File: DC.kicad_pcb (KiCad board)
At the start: 4 copper layers, 196.5 x 181.5 mm, 87 parts, among them J1 348302001, J2 348302001, J3 757570141, J4 PPTC021LFBN-RC, U6 MCP2551-I-P, U7 NUCLEO-F302R8

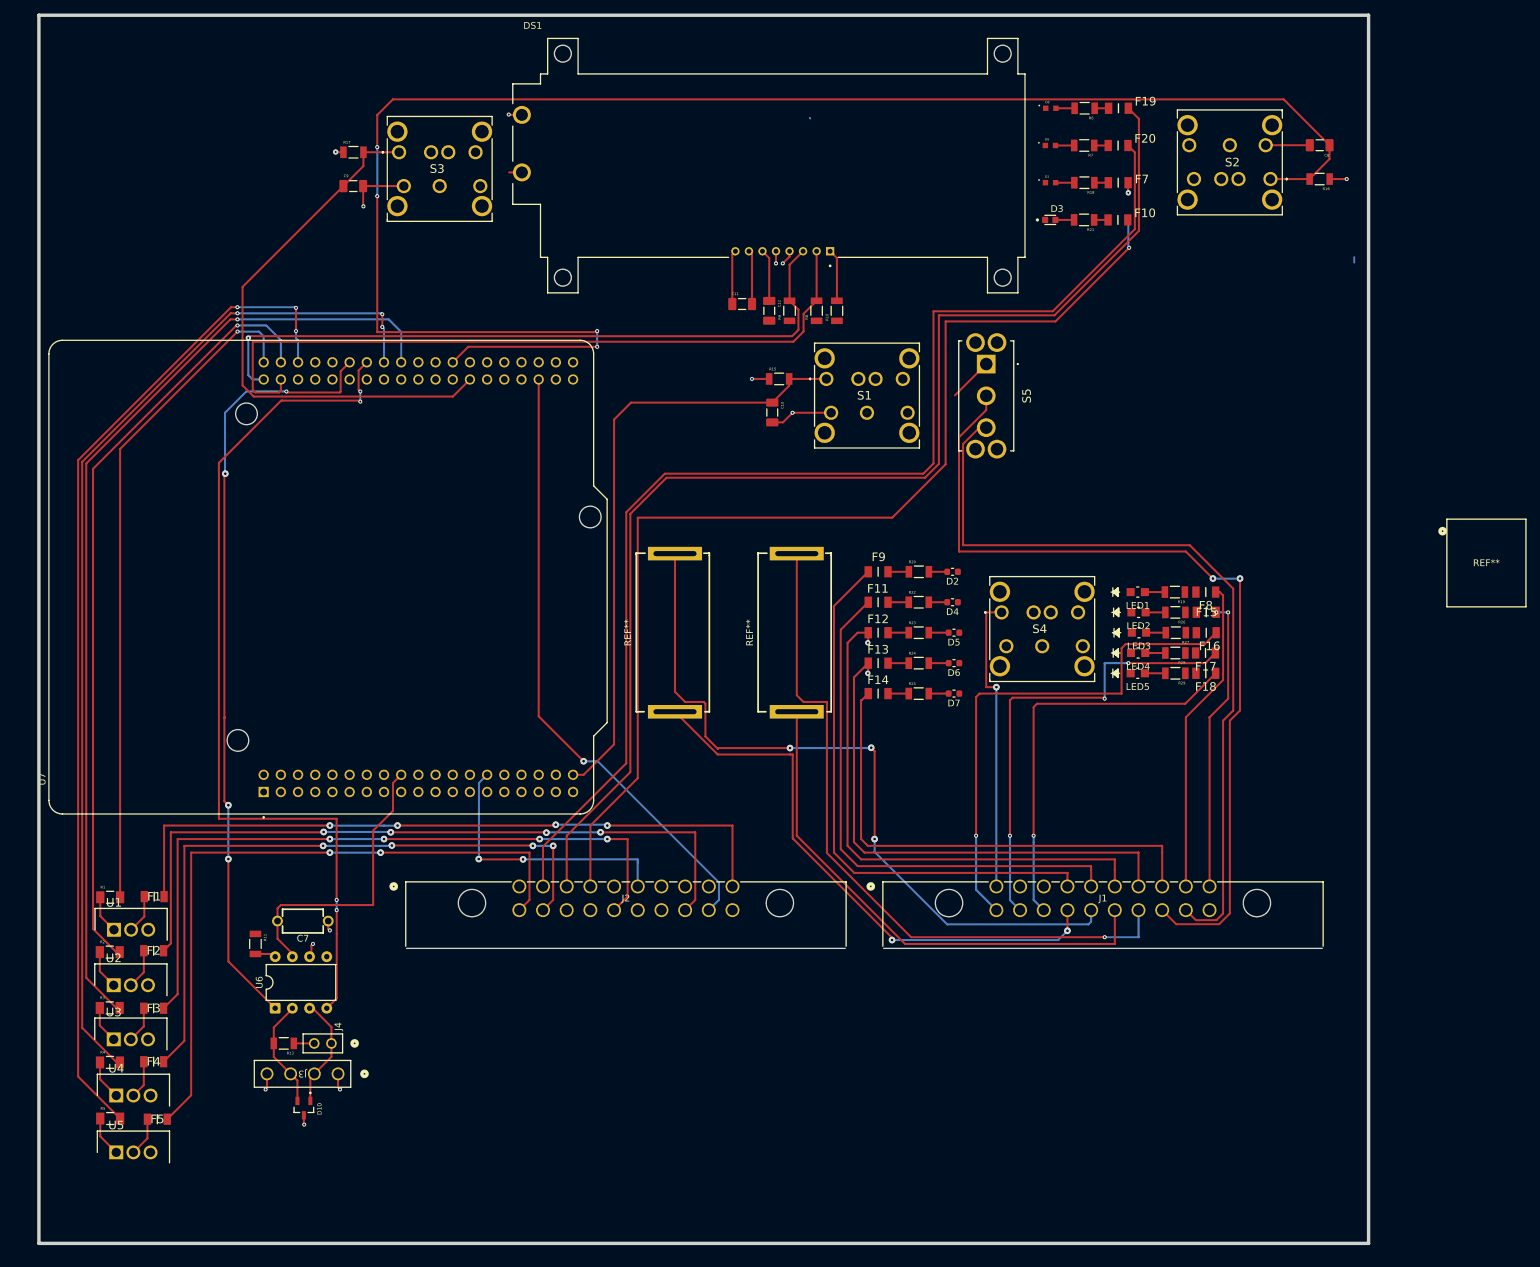
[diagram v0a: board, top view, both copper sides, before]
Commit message: Updated pcb with new routing and gear select. Still errors to correct
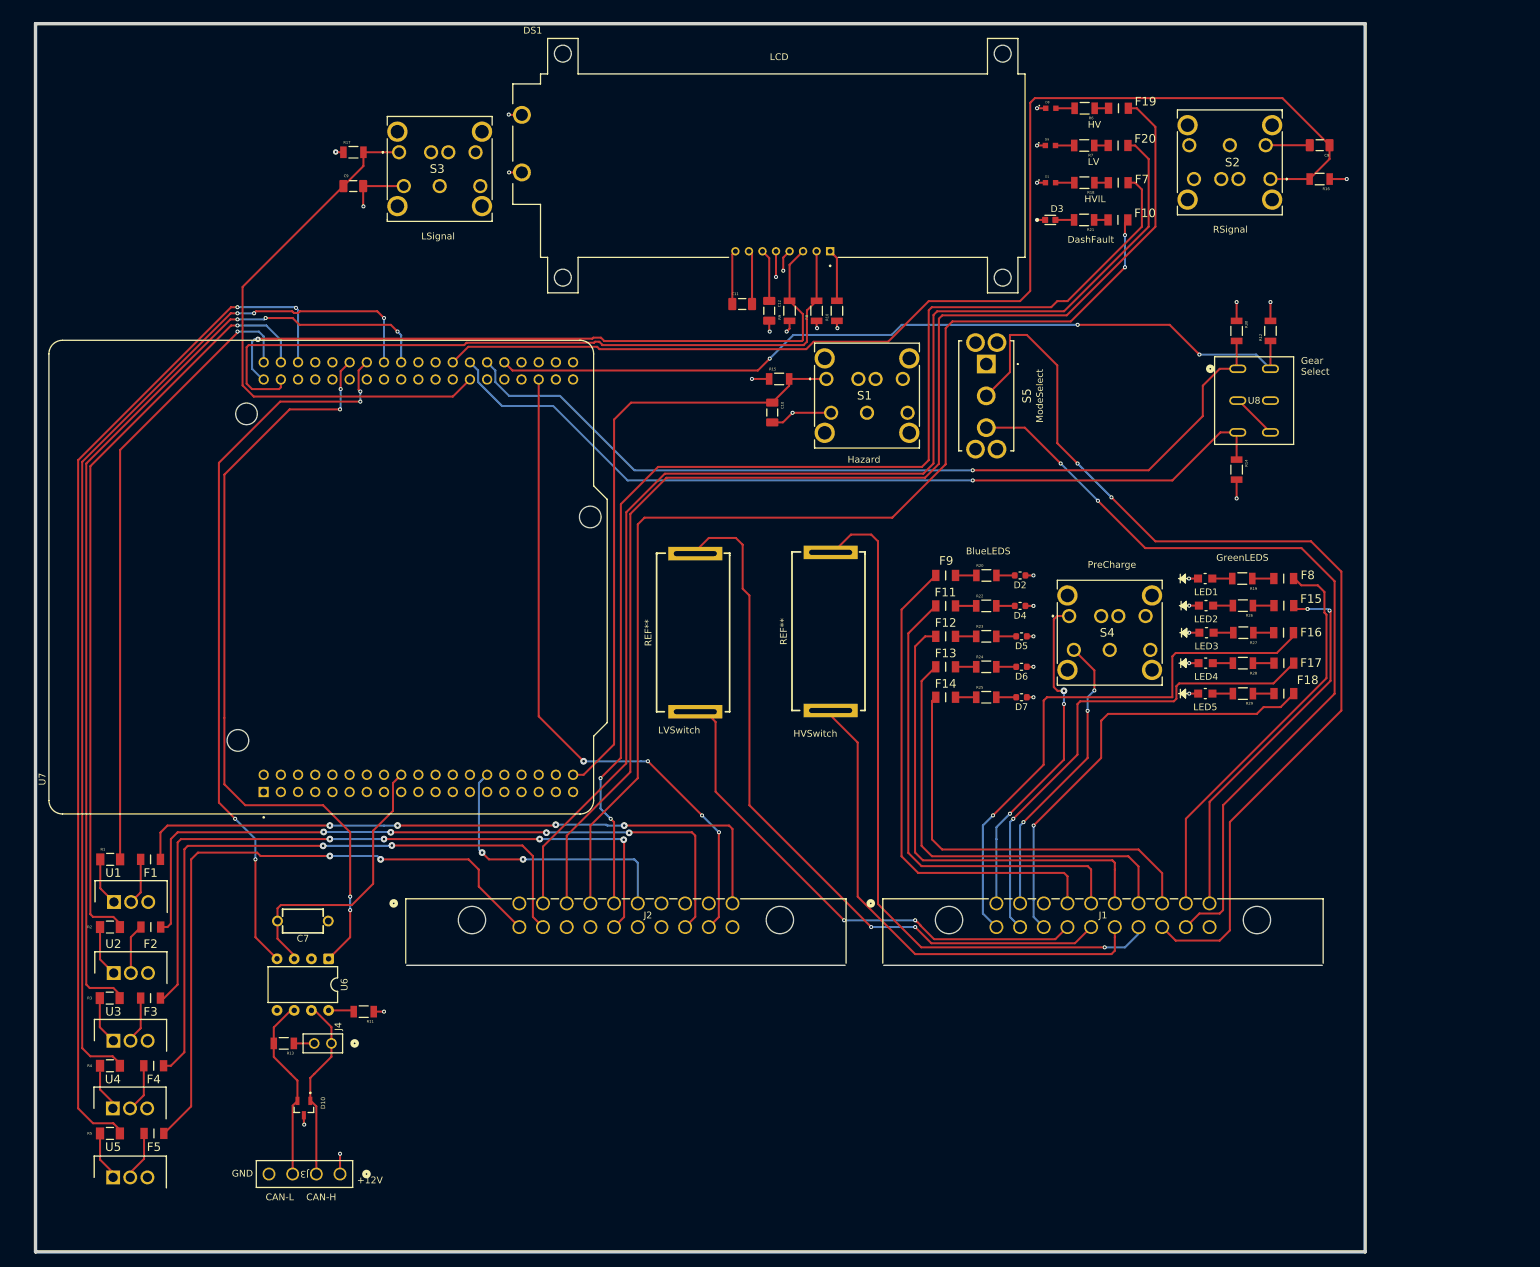
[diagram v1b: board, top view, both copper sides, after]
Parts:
- removed the REF** at (285.0, 92.0)
- added R12: RC1206FR-0710KL, MiscellaneousLibrary:RESC3116X65N, F.Cu at (255.5, 62.4)
- added R14: RC1206FR-0710KL, MiscellaneousLibrary:RESC3116X65N, F.Cu at (250.5, 82.9)
- added R30: RC1206FR-0710KL, MiscellaneousLibrary:RESC3116X65N, F.Cu at (250.5, 62.4)
- added U8: 100DP6T1B1M1QEH, MiscellaneousLibrary:TO_1M1QEH_EWI, F.Cu at (250.7, 68.0)
- moved R11 18.9 mm to (121.5, 163.0), turned to 180 degrees
- moved J3 14.8 mm to (118.0, 187.0)
- moved F18 11.9 mm to (257.5, 116.0)
- moved F8 11.7 mm to (257.5, 99.0)
- moved F17 11.7 mm to (257.5, 111.5)
- moved F15 11.5 mm to (257.5, 103.0)
- moved F16 11.4 mm to (257.4, 107.0)
- moved U6 10.8 mm to (116.3, 155.2), turned to -90 degrees
- moved LED5 10.4 mm to (245.9, 116.0)
- moved R29 10.4 mm to (251.4, 116.0)
- moved LED1 10.2 mm to (245.9, 99.0)
- moved R19 10.2 mm to (251.3, 99.0)
- moved LED4 10.1 mm to (245.9, 111.5)
- moved R28 10.1 mm to (251.4, 111.5)
- moved R26 10.0 mm to (251.4, 103.0)
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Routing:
- net /HVILActive: track 1.52 -> 176.0 mm, vias 1 -> 2
- net /Neutral: track 0.00 -> 131.6 mm, vias 0 -> 1
- net /Drive: track 0.00 -> 128.7 mm, vias 0 -> 1
- net /Reverse: track 0.00 -> 123.3 mm, vias 0 -> 3
- net /RSignalLightIn: track 245.8 -> 177.2 mm, vias 4 -> 0
- net /From_PreChargeBtn: track 0.00 -> 43.3 mm, vias 0 -> 3
- net /To_ModeSelect: track 129.5 -> 151.9 mm
- net /CAN_RX: track 129.8 -> 108.2 mm
- net GND: track 35.3 -> 49.8 mm, vias 7 -> 22
- net /GreenLED1: track 46.6 -> 60.1 mm
- net /GreenLED2: track 43.4 -> 56.3 mm
- net +3.3V: track 9.92 -> 22.4 mm, vias 4 -> 10
- net /BlueLED5: track 72.9 -> 61.8 mm
- net /CAN_H: track 16.4 -> 27.1 mm
- net /BlueLED4: track 76.5 -> 66.1 mm, vias 1 -> 0
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- added copper zone on In1.Cu, net +3.3V
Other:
- board text added: "+12V"
- board text added: "BlueLEDS"
- board text added: "CAN-H"
- board text added: "CAN-L"
- board text added: "DashFault"
- board text added: "GND"
- board text added: "Gear Select"
- board text added: "GreenLEDS"
- board text added: "HV"
- board text added: "HVIL"
- board text added: "HVSwitch"
- board text added: "Hazard"
- board text added: "LCD"
- board text added: "LSignal"
- board text added: "LV"
- board text added: "LVSwitch"
- board text added: "ModeSelect"
- board text added: "PreCharge"
- board text added: "RSignal"

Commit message: VCU revisions, last review still to be done
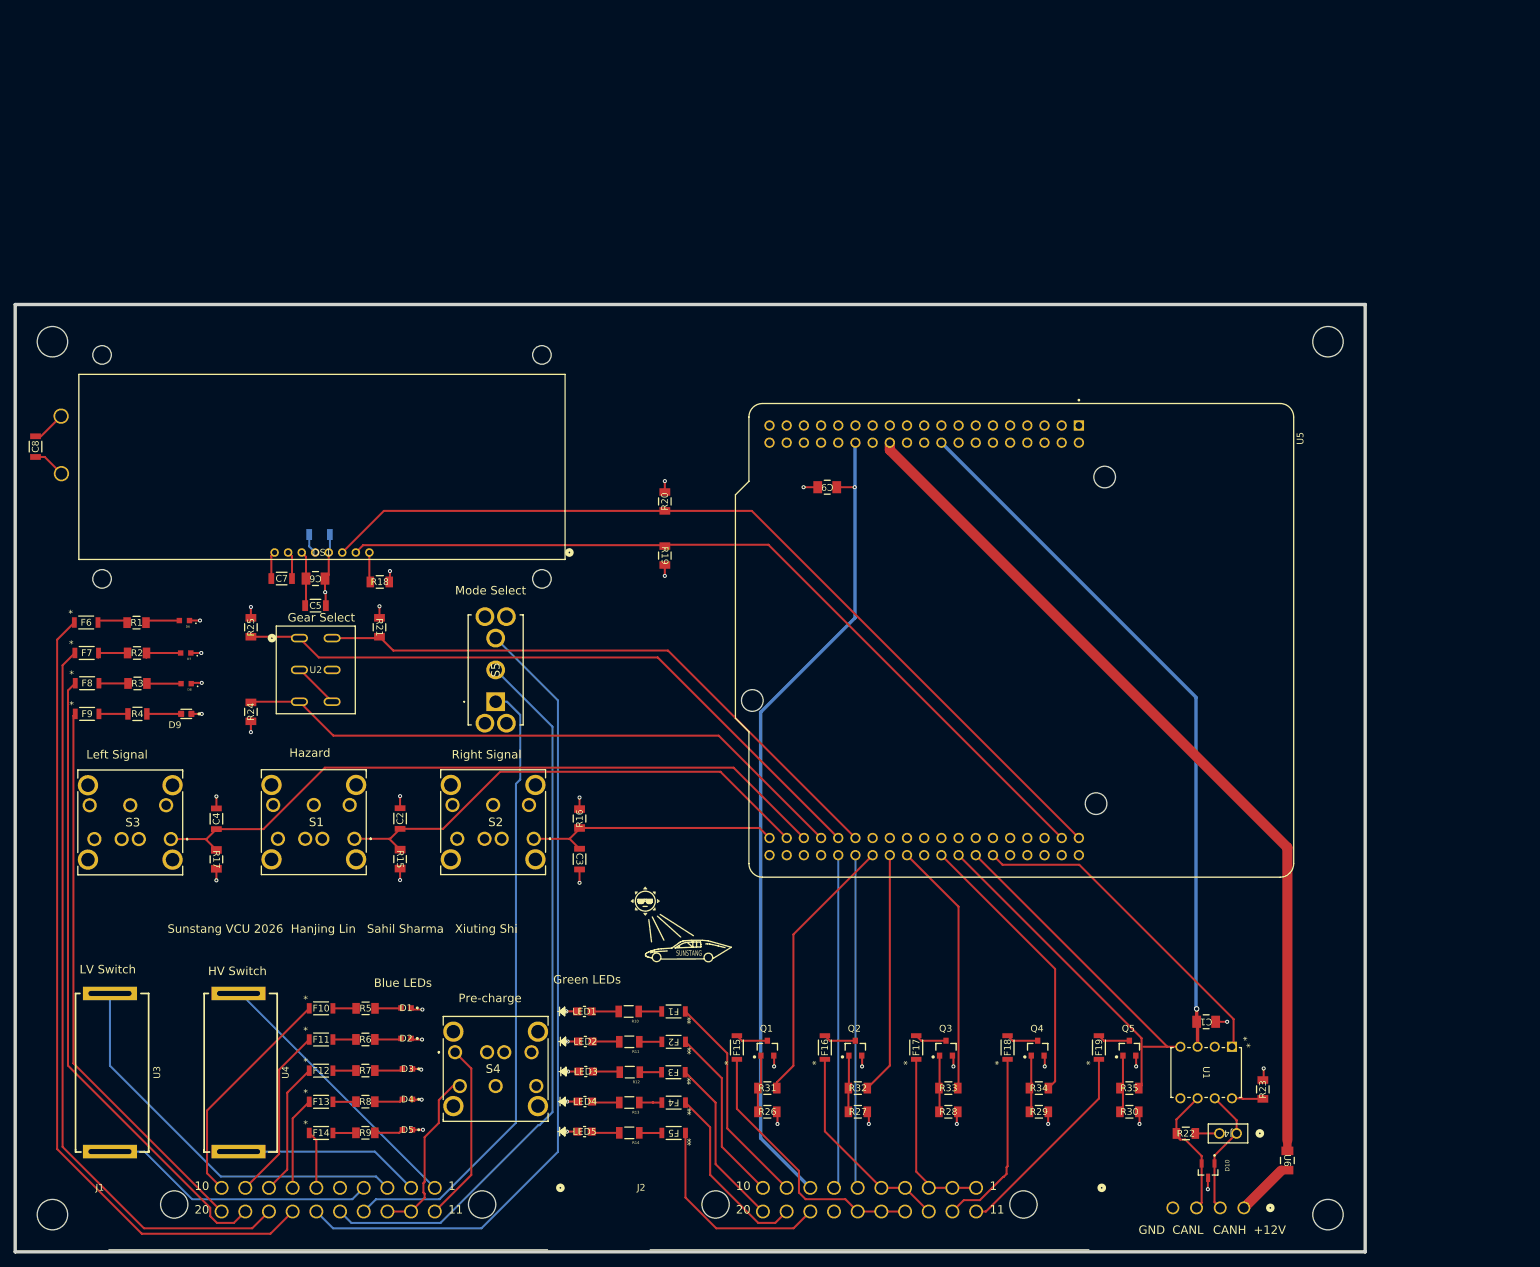
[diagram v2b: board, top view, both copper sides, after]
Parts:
- removed C11: CL31B105KAHNNNE, Capacitor_SMD:CAPC3216X180N
- removed C12: C3216X7R2A474K160AA, Capacitor_SMD:CAPC3216X180N
- removed the F1 at (90.0, 140.5)
- removed the F2 at (90.0, 150.5)
- removed the F3 at (90.0, 161.0)
- removed the F4 at (90.5, 171.0)
- removed the F5 at (90.5, 181.0)
- removed the R18 at (228.0, 40.5)
- removed the R4 at (84.0, 171.0)
- removed the R5 at (84.0, 181.0)
- removed the R6 at (228.0, 29.5)
- removed the R7 at (228.0, 35.0)
- removed the REF** at (170.5, 107.0)
- removed the REF** at (190.5, 106.8)
- removed the U1 at (84.6, 146.8)
- removed the U5 at (84.5, 187.5)
- removed U8: 100DP6T1B1M1QEH, MiscellaneousLibrary:TO_1M1QEH_EWI
- added C1: C1206C104K5RACTU, DriverControlsLib:CAPC340180_88N_KEM, F.Cu at (246.0, 164.5)
- added C5: CL31B105KAHNNNE, DriverControlsLib:CAP_CL31_SAM, F.Cu at (114.4, 103.0)
- added C6: C1206C104K5RACTU, DriverControlsLib:CAPC340180_88N_KEM, F.Cu at (114.4, 99.0)
- added C8: CL31B225KBHNNNE, DriverControlsLib:CAP_CL31_SAM, F.Cu at (73.0, 79.5)
- added C8: CL31B225KBHNNNE, DriverControlsLib:CAP_CL31_SAM, B.Cu at (115.0, 92.5)
- added C9: C1206C104K5RACTU, DriverControlsLib:CAPC340180_88N_KEM, F.Cu at (190.0, 85.5)
- added F15: 0466.125NR, DriverControlsLib:0466Series_LTF, F.Cu at (176.7, 168.3)
- added F16: 0466.125NR, DriverControlsLib:0466Series_LTF, F.Cu at (189.7, 168.3)
- added F17: 0466.125NR, DriverControlsLib:0466Series_LTF, F.Cu at (203.2, 168.3)
- added F18: 0466.125NR, DriverControlsLib:0466Series_LTF, F.Cu at (216.7, 168.3)
- added F19: 0466.125NR, DriverControlsLib:0466Series_LTF, F.Cu at (230.2, 168.3)
- added Q1: BSS806NE, DriverControlsLib:SOT95P240X110-3N-1-V1, F.Cu at (181.2, 168.4)
- added Q2: BSS806NE, DriverControlsLib:SOT95P240X110-3N-1-V1, F.Cu at (194.2, 168.4)
- added Q3: BSS806NE, DriverControlsLib:SOT95P240X110-3N-1-V1, F.Cu at (207.6, 168.4)
- added Q4: BSS806NE, DriverControlsLib:SOT95P240X110-3N-1-V1, F.Cu at (221.1, 168.4)
- added Q5: BSS806NE, DriverControlsLib:SOT95P240X110-3N-1-V1, F.Cu at (234.7, 168.4)
- added R26: RC1206FR-0710KL, DriverControlsLib:RC1206N_YAG, F.Cu at (181.2, 177.8)
- added R27: RC1206FR-0710KL, DriverControlsLib:RC1206N_YAG, F.Cu at (194.5, 177.8)
- added R28: RC1206FR-0710KL, DriverControlsLib:RC1206N_YAG, F.Cu at (207.9, 177.8)
- added R29: RC1206FR-0710KL, DriverControlsLib:RC1206N_YAG, F.Cu at (221.3, 177.8)
- added R30: RC1206FR-0710KL, DriverControlsLib:RC1206N_YAG, F.Cu at (234.7, 177.8)
- added R31: RC1206JR-07120RL, DriverControlsLib:RC1206N_YAG, F.Cu at (181.2, 174.3)
- added R32: RC1206JR-07120RL, DriverControlsLib:RC1206N_YAG, F.Cu at (194.5, 174.3)
- added R33: RC1206JR-07120RL, DriverControlsLib:RC1206N_YAG, F.Cu at (207.9, 174.3)
- added R34: RC1206JR-07120RL, DriverControlsLib:RC1206N_YAG, F.Cu at (221.3, 174.3)
- added R35: RC1206JR-07120RL, DriverControlsLib:RC1206N_YAG, F.Cu at (234.7, 174.3)
- added REF**: MountingHole_4.5mm, MountingHole:MountingHole_4.5mm, F.Cu at (264.0, 64.0)
- added REF**: MountingHole_4.5mm, MountingHole:MountingHole_4.5mm, F.Cu at (75.5, 193.0)
- added REF**: MountingHole_4.5mm, MountingHole:MountingHole_4.5mm, F.Cu at (264.0, 193.0)
- added REF**: MountingHole_4.5mm, MountingHole:MountingHole_4.5mm, F.Cu at (75.5, 64.0)
- added U6: C1F 3, DriverControlsLib:C1_BEL, F.Cu at (258.0, 185.0)
- C2: renamed from C10; footprint Capacitor_SMD:CAPC3216X180N -> DriverControlsLib:CAP_CL31_SAM
- C3: renamed from C8; footprint Capacitor_SMD:CAPC3216X180N -> DriverControlsLib:CAP_CL31_SAM
- C4: renamed from C9; footprint Capacitor_SMD:CAPC3216X180N -> DriverControlsLib:CAP_CL31_SAM
- C7: value C -> CL31B105KAHNNNE; footprint DriverControlsLib:CAP-TH_L6.0-W3.5-P7.50-D1.0 -> DriverControlsLib:CAP_CL31_SAM
- D1: renamed from D2; footprint Fuse:Fuse_0603_1608Metric -> DriverControlsLib:LED_LTST-C_LTO
- D2: renamed from D4; footprint Fuse:Fuse_0603_1608Metric -> DriverControlsLib:LED_LTST-C_LTO
- D3: renamed from D5; footprint Fuse:Fuse_0603_1608Metric -> DriverControlsLib:LED_LTST-C_LTO
- D4: renamed from D6; footprint Fuse:Fuse_0603_1608Metric -> DriverControlsLib:LED_LTST-C_LTO
- D5: renamed from D7; footprint Fuse:Fuse_0603_1608Metric -> DriverControlsLib:LED_LTST-C_LTO
- D6: renamed from D9; footprint LED_SMD:LEDM1608X80 -> DriverControlsLib:LEDM1608X80
- D7: renamed from D8; footprint LED_SMD:LEDM1608X80 -> DriverControlsLib:LEDM1608X80
- D8: renamed from D1; footprint LED_SMD:LEDM1608X80 -> DriverControlsLib:LEDM1608X80
- D9: renamed from D3; footprint LED_SMD:LEDC1608X65N -> DriverControlsLib:LEDC1608X65N
- DS1: footprint Display:LCD_NHD-C0220BIZ-FSW-FBW-3V3M -> DriverControlsLib:NHD-C0220BIZ-FSW-FBW-3V3M_NDI
- F1: renamed from F8; footprint Fuse:FUSC3215X66N -> DriverControlsLib:0466Series_LTF
- F10: renamed from F9; footprint Fuse:FUSC3215X66N -> DriverControlsLib:0466Series_LTF
- F11, F12, F13, F14: footprint Fuse:FUSC3215X66N -> DriverControlsLib:0466Series_LTF
- F2: renamed from F15; footprint Fuse:FUSC3215X66N -> DriverControlsLib:0466Series_LTF
- F3: renamed from F16; footprint Fuse:FUSC3215X66N -> DriverControlsLib:0466Series_LTF
- F4: renamed from F17; footprint Fuse:FUSC3215X66N -> DriverControlsLib:0466Series_LTF
- F5: renamed from F18; footprint Fuse:FUSC3215X66N -> DriverControlsLib:0466Series_LTF
- F6: renamed from F20; footprint Fuse:FUSC3215X66N -> DriverControlsLib:0466Series_LTF
- F7: renamed from F19; footprint Fuse:FUSC3215X66N -> DriverControlsLib:0466Series_LTF
- F8: renamed from F7; footprint Fuse:FUSC3215X66N -> DriverControlsLib:0466Series_LTF
- F9: renamed from F10; footprint Fuse:FUSC3215X66N -> DriverControlsLib:0466Series_LTF
- J1, J2: footprint Connector_Molex:CONN_SD-34829-001_20_ST_MOL -> DriverControlsLib:CONN_SD-34829-001_20_ST_MOL; moved to B.Cu
- J3: footprint Connector_Molex:CONN_SD-75757-010_1X4_F11p20_MOL -> DriverControlsLib:CONN_SD-75757-010_1X4_F11p20_MOL; moved to B.Cu
- J4: footprint Connector:CONN2_LFBN-RC_SUL -> DriverControlsLib:CONN2_LFBN-RC_SUL
- LED1, LED2, LED3, LED4, LED5: footprint LED_SMD:LED_LTST-C170GKT_LTO -> DriverControlsLib:LED_LTST-C170GKT_LTO
- R1, R2, R3: value 220Ω -> RC1206FR-07665RL; footprint Resistor_SMD:RESC3216X70N -> DriverControlsLib:RC1206N_YAG
- R10: renamed from R19; footprint Resistor_SMD:RESC3116X65N -> DriverControlsLib:RESC3116X65N
- R11: renamed from R26; footprint Resistor_SMD:RESC3116X65N -> DriverControlsLib:RESC3116X65N
- R12: renamed from R27; footprint Resistor_SMD:RESC3116X65N -> DriverControlsLib:RESC3116X65N
- R13: renamed from R28; footprint Resistor_SMD:RESC3116X65N -> DriverControlsLib:RESC3116X65N
- R14: renamed from R29; footprint Resistor_SMD:RESC3116X65N -> DriverControlsLib:RESC3116X65N
- R15, R16, R17: footprint Resistor_SMD:RESC3116X65N -> DriverControlsLib:RC1206N_YAG
- R18: renamed from R10; footprint Resistor_SMD:RESC3116X65N -> DriverControlsLib:RC1206N_YAG
- R19: renamed from R8; footprint Resistor_SMD:RESC3116X65N -> DriverControlsLib:RC1206N_YAG
- R20: renamed from R9; footprint Resistor_SMD:RESC3116X65N -> DriverControlsLib:RC1206N_YAG
- R21: renamed from R12; footprint MiscellaneousLibrary:RESC3116X65N -> DriverControlsLib:RC1206N_YAG
- R22: renamed from R13; footprint Resistor_SMD:RESC3116X65N -> DriverControlsLib:RC1206N_YAG
- R23: renamed from R11; footprint Resistor_SMD:RESC3116X65N -> DriverControlsLib:RC1206N_YAG
- R24: renamed from R14; footprint MiscellaneousLibrary:RESC3116X65N -> DriverControlsLib:RC1206N_YAG
- R25: renamed from R30; footprint MiscellaneousLibrary:RESC3116X65N -> DriverControlsLib:RC1206N_YAG
- R4: renamed from R21; footprint Resistor_SMD:RESC3116X65N -> DriverControlsLib:RES_RC1206_YAG
- R5: renamed from R20; footprint Resistor_SMD:RESC3116X65N -> DriverControlsLib:RC1206N_YAG
- R6: renamed from R22; footprint Resistor_SMD:RESC3116X65N -> DriverControlsLib:RC1206N_YAG
- R7: renamed from R23; footprint Resistor_SMD:RESC3116X65N -> DriverControlsLib:RC1206N_YAG
- R8: renamed from R24; footprint Resistor_SMD:RESC3116X65N -> DriverControlsLib:RC1206N_YAG
- R9: renamed from R25; footprint Resistor_SMD:RESC3116X65N -> DriverControlsLib:RC1206N_YAG
- S1, S2, S3, S4: footprint Button_Switch_SMD:LP6OA2ASRG -> DriverControlsLib:LP6OA2ASRG
- S5: footprint Button_Switch_SMD:100SP1T8B13VS2REH -> DriverControlsLib:100SP1T8B13VS2REH
- U1: renamed from U6; footprint Package_DIP:DIP-8_W7.62mm -> DriverControlsLib:PDIP8_300MC_MCH
- U2: value ~ -> 100DP6T1B1M1QEH; footprint Battery:TO254P470X1016X2019-3P -> DriverControlsLib:TO_1M1QEH_EWI
- U3: footprint Battery:TO254P470X1016X2019-3P -> DriverControlsLib:LV_Switch
- U4: footprint Battery:TO254P470X1016X2019-3P -> DriverControlsLib:HV_Switch
- U5: renamed from U7; footprint Module:MODULE_NUCLEO-F302R8 -> DriverControlsLib:MODULE_NUCLEO-F302R8
- moved F7 172.4 mm to (80.6, 110.0), turned to 0 degrees
- moved F8 169.4 mm to (80.6, 114.5), turned to 0 degrees
- moved F9 168.9 mm to (80.6, 119.0), turned to 0 degrees
- moved F6 168.0 mm to (80.5, 105.5), turned to 0 degrees
- moved R4 157.8 mm to (88.1, 119.0), turned to 0 degrees
- moved R25 152.1 mm to (104.8, 106.2), turned to 90 degrees
- moved C3 152.0 mm to (153.4, 140.5), turned to -90 degrees
- moved D7 151.1 mm to (95.2, 110.0), turned to 180 degrees
- moved R24 150.0 mm to (104.8, 118.7), turned to 90 degrees
- moved D8 147.6 mm to (95.3, 114.5), turned to 180 degrees
- moved D9 147.1 mm to (95.3, 119.0), turned to 180 degrees
- moved S2 146.2 mm to (146.6, 137.5)
- moved D6 146.0 mm to (95.0, 105.2), turned to 180 degrees
- moved R16 144.5 mm to (153.4, 134.5), turned to 90 degrees
- moved R21 138.8 mm to (123.8, 106.2), turned to -90 degrees
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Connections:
- C7 pad 1: GND -> Net-(DS1-C1-)
- C7 pad 2: /CANTransceiver5V -> Net-(DS1-C1+)
- D1 pad 2: Net-(D2-Pad2) -> Net-(D1-Pad2)
- D2 pad 2: Net-(D4-Pad2) -> Net-(D2-Pad2)
- D3 pad 2: Net-(D5-Pad2) -> Net-(D3-Pad2)
- D4 pad 2: Net-(D6-Pad2) -> Net-(D4-Pad2)
- D5 pad 2: Net-(D7-Pad2) -> Net-(D5-Pad2)
- D6 pad A: Net-(D9-PadA) (its old number) -> Net-(D6-PadA)
- D7 pad A: Net-(D8-PadA) -> Net-(D7-PadA)
- D8 pad A: Net-(D1-PadA) -> Net-(D8-PadA)
- DS1 pad 1: Net-(DS1A-RST) -> Net-(DS1-ST)
- DS1 pad 7: Net-(DS1A-C1P) -> Net-(DS1-C1+)
- DS1 pad 8: Net-(DS1A-C1N) -> Net-(DS1-C1-)
- F10 pad 2: Net-(F9-Pad2) (its old number) -> Net-(F10-Pad2)
- F6 pad 2: Net-(F20-Pad2) -> Net-(F6-Pad2)
- F7 pad 2: Net-(F19-Pad2) -> Net-(F7-Pad2)
- F8 pad 2: Net-(F7-Pad2) -> Net-(F8-Pad2)
- J1 pad 1: /To_PreChargeBtn -> /HVSwitch+
- J1 pad 10: /GreenLED2 -> /BlueLED1
- J1 pad 11: /GreenLED3 -> /To_PreChargeBtn
- J1 pad 12: /GreenLED4 -> /Enable
- J1 pad 13: /GreenLED5 -> /Enable
- J1 pad 14: /LVSwitch+ -> /ChargeMode
- J1 pad 15: /LVSwitch- -> /To_ModeSelect
- J1 pad 16: /HVSwitch+ -> /ReadyMode
- J1 pad 17: /HVSwitch- -> /LVActive
- J1 pad 18: /To_ModeSelect -> /HVActive
- J1 pad 19: /ReadyMode -> /HVILActive
- J1 pad 2: /From_PreChargeBtn -> /HVSwitch-
- J1 pad 20: GND -> /DashFaultIndicator
- J1 pad 3: /Enable -> /LVSwitch+
- J1 pad 4: /BlueLED1 -> /LVSwitch-
- J1 pad 5: /BlueLED2 -> GND
- J1 pad 6: /BlueLED3 -> /BlueLED5
- J1 pad 8: /BlueLED5 -> /BlueLED3
- J1 pad 9: /GreenLED1 -> /BlueLED2
- J2 pad 1: /ChargeMode -> /LSignalLightNeg
- J2 pad 10: /BrakeLightNeg -> /GreenLED2
- J2 pad 13: /LSignalLightNeg -> /RSignalLightNeg
- J2 pad 14: /LSignalLightNeg -> /BrakeLightNeg
- J2 pad 15: /LSignalLightNeg -> /BrakeLightNeg
- J2 pad 16: /RSignalLightNeg -> /BrakeLightNeg
- J2 pad 17: /RSignalLightNeg -> GND
- J2 pad 18: /RSignalLightNeg -> /GreenLED5
- J2 pad 19: /ThermalShutoff -> /GreenLED4
- J2 pad 2: /LVActive -> /LSignalLightNeg
- J2 pad 20: GND -> /GreenLED3
- J2 pad 3: /HVActive -> /LSignalLightNeg
- J2 pad 4: /DashFaultIndicator -> /RSignalLightNeg
- J2 pad 5: /HVILActive -> /RSignalLightNeg
- J2 pad 6: /AccelIn -> /ThermalShutoff
- J2 pad 7: /BrakeLightIn -> /BrakePedalIn
- J2 pad 8: /BrakeLightNeg -> /AccelIn
- J2 pad 9: /BrakeLightNeg -> /GreenLED1
- R1 pad 1: Net-(U1-G) -> Net-(D6-PadA)
- R1 pad 2: /BrakeLightOut -> Net-(F6-Pad2)
- R15 pad 1: +3.3V -> /HazardIn
- R15 pad 2: /HazardIn -> +3.3V
- R16 pad 1: +3.3V -> /RSignalLightIn
- R16 pad 2: /RSignalLightIn -> +3.3V
- R17 pad 1: +3.3V -> /LSignalLightIn
- R17 pad 2: /LSignalLightIn -> +3.3V
- R18 pad 1: GND -> Net-(DS1-ST)
- R18 pad 2: Net-(DS1A-RST) -> GND
- R19 pad 1: +3.3V -> /I2C1_CLK
- R19 pad 2: /I2C1_CLK -> +3.3V
- R2 pad 1: Net-(U2-G) -> Net-(D7-PadA)
- R2 pad 2: /RSignalLightOut -> Net-(F7-Pad2)
- R20 pad 1: +3.3V -> /I2C1_SDA
- R20 pad 2: /I2C1_SDA -> +3.3V
- R21 pad 1: /Reverse -> +3.3V
- R21 pad 2: +3.3V -> /Reverse
- R22 pad 1: Net-(J4-Pad2) -> /CAN_L
- R22 pad 2: /CAN_L -> Net-(J4-Pad2)
- R23 pad 1: GND -> Net-(U1-RS)
- R23 pad 2: Net-(U6-Rs) -> GND
- R24 pad 1: /Drive -> +3.3V
- R24 pad 2: +3.3V -> /Drive
- R25 pad 1: +3.3V -> /Neutral
- R25 pad 2: /Neutral -> +3.3V
- R3 pad 1: Net-(U3-G) -> Net-(D8-PadA)
- R3 pad 2: /LSignalLightOut -> Net-(F8-Pad2)
- R5 pad 1: Net-(F9-Pad2) (its old number) -> Net-(D1-Pad2)
- R5 pad 2: Net-(D2-Pad2) -> Net-(F10-Pad2)
- R6 pad 1: Net-(F11-Pad2) -> Net-(D2-Pad2)
- R6 pad 2: Net-(D4-Pad2) -> Net-(F11-Pad2)
- R7 pad 1: Net-(F12-Pad2) -> Net-(D3-Pad2)
- R7 pad 2: Net-(D5-Pad2) -> Net-(F12-Pad2)
- R8 pad 1: Net-(F13-Pad2) -> Net-(D4-Pad2)
- R8 pad 2: Net-(D6-Pad2) -> Net-(F13-Pad2)
- R9 pad 1: Net-(F14-Pad2) -> Net-(D5-Pad2)
- R9 pad 2: Net-(D7-Pad2) -> Net-(F14-Pad2)
- S1 pad MH1: unconnected-(S1-PadMH1) -> GND
- S1 pad MH2: unconnected-(S1-PadMH2) -> GND
- S1 pad MH3: unconnected-(S1-PadMH3) -> GND
- S1 pad MH4: unconnected-(S1-PadMH4) -> GND
- S2 pad MH1: unconnected-(S2-PadMH1) -> GND
- S2 pad MH2: unconnected-(S2-PadMH2) -> GND
- S2 pad MH3: unconnected-(S2-PadMH3) -> GND
- S2 pad MH4: unconnected-(S2-PadMH4) -> GND
- S3 pad MH1: unconnected-(S3-PadMH1) -> GND
- S3 pad MH2: unconnected-(S3-PadMH2) -> GND
- S3 pad MH3: unconnected-(S3-PadMH3) -> GND
- S3 pad MH4: unconnected-(S3-PadMH4) -> GND
- S4 pad 2: /From_PreChargeBtn -> /Enable
- S4 pad MH1: unconnected-(S4-PadMH1) -> GND
- S4 pad MH2: unconnected-(S4-PadMH2) -> GND
- S4 pad MH3: unconnected-(S4-PadMH3) -> GND
- S4 pad MH4: unconnected-(S4-PadMH4) -> GND
- S5 pad 1: unconnected-(S5-NC-Pad1) -> /ChargeMode
- S5 pad 4: unconnected-(S5-MH1-Pad4) -> GND
- S5 pad 5: unconnected-(S5-MH2-Pad5) -> GND
- S5 pad 6: unconnected-(S5-MH3-Pad6) -> GND
- S5 pad 7: unconnected-(S5-MH4-Pad7) -> GND
- U1 pad 8: Net-(U6-Rs) -> Net-(U1-RS)
- U2 pad 1: Net-(U2-G) -> /Reverse
- U2 pad 2: Net-(U2-D) -> GND
- U2 pad 3: GND -> Net-(U2-Pad3)
- U3 pad 1: Net-(U3-G) -> /LVSwitch+
- U3 pad 2: Net-(U3-D) -> /LVSwitch-
- U4 pad 1: Net-(U4-G) -> /HVSwitch+
- U4 pad 2: Net-(U4-D) -> /HVSwitch-
- U5 pad CN10_16: /DRLRightOut -> /DRLLeftOut
- U5 pad CN10_18: /LSignalLightOut -> /DRLRightOut
- U5 pad CN10_2: /BrakeLightOut -> unconnected-(U5B-PC8-PadCN10_2)
- U5 pad CN10_20: unconnected-(U7B-GND_CN10_20-PadCN10_20) -> GND
- U5 pad CN10_21: /BrakePedalIn -> unconnected-(U5B-PA9-PadCN10_21)
- U5 pad CN10_22: unconnected-(U7B-PB2-PadCN10_22) -> /LSignalLightOut
- U5 pad CN10_24: /RSignalLightIn -> /RSignalLightOut
- U5 pad CN10_25: /LSignalLightIn -> unconnected-(U5B-PB10-PadCN10_25)
- U5 pad CN10_26: /Drive -> /BrakeLightOut
- U5 pad CN10_27: unconnected-(U7B-PB4-PadCN10_27) -> /Reverse
- U5 pad CN10_28: /Neutral -> /ThermalShutoff
- U5 pad CN10_29: unconnected-(U7B-PB5-PadCN10_29) -> /Neutral
- U5 pad CN10_30: /Reverse -> /BrakePedalIn
- U5 pad CN10_31: unconnected-(U7B-PB3-PadCN10_31) -> /Drive
- U5 pad CN10_33: /ThermalShutoff -> /LSignalLightIn
- U5 pad CN10_35: /UART_TX -> /HazardIn
- U5 pad CN10_37: /UART_RX -> /RSignalLightIn
- U5 pad CN10_4: /RSignalLightOut -> unconnected-(U5B-PC6-PadCN10_4)
- U5 pad CN10_6: /DRLLeftOut -> unconnected-(U5B-PC5-PadCN10_6)
- U5 pad CN7_32: /DIExtra1 -> unconnected-(U5A-PA4-PadCN7_32)
- U5 pad CN7_34: /DIExtra2 -> unconnected-(U5A-PB0-PadCN7_34)
- U5 pad CN7_36: /DOExtra1 -> unconnected-(U5A-PC1-PadCN7_36)
- U5 pad CN7_38: /HazardIn -> unconnected-(U5A-PC0-PadCN7_38)
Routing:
- net /RSignalLightIn: track 177.2 -> 38.3 mm
- net Net-(U5A-VIN): track 0.00 -> 129.0 mm
- net /DRLRightOut: track 154.5 -> 41.8 mm, vias 3 -> 0
- net /DRLLeftOut: track 153.6 -> 45.8 mm, vias 2 -> 0
- net /LSignalLightOut: track 143.6 -> 37.6 mm, vias 3 -> 0
- net /ChargeMode: track 0.00 -> 92.9 mm
- net /DashFaultIndicator: track 165.6 -> 82.7 mm, vias 2 -> 0
- net /HVILActive: track 176.0 -> 94.2 mm, vias 2 -> 0
- net /AccelIn: track 41.8 -> 121.6 mm, vias 2 -> 1
- net /HVActive: track 189.1 -> 110.3 mm
- net /LSignalLightNeg: track 104.3 -> 26.8 mm, vias 4 -> 0
- net /RSignalLightOut: track 112.6 -> 35.8 mm, vias 1 -> 0
- net /HVSwitch-: track 104.1 -> 27.7 mm, vias 1 -> 0
- net /RSignalLightNeg: track 106.6 -> 30.9 mm, vias 4 -> 0
- net /DRLRightNeg: track 97.4 -> 27.3 mm, vias 2 -> 0
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- removed copper zone on In1.Cu, net (none)
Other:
- board size 196.5 x 181.5 mm -> 199.5 x 140 mm
- board text added: "1"
- board text added: "10"
- board text added: "11"
- board text added: "20"
- board text added: "Blue LEDs"
- board text added: "CANH"
- board text added: "CANL"
- board text added: "Green LEDs"
- board text added: "HV Switch"
- board text added: "LV Switch"
- board text added: "Left Signal"
- board text added: "Mode Select"
- board text added: "Pre-charge"
- board text added: "Right Signal"
- board text added: "SUNSTANG"
- board text added: "Sunstang VCU 2026 Hanjing Lin Sahil Sharma Xiuting Shi"
- board text removed: "BlueLEDS"
- board text removed: "CAN-H"
- board text removed: "CAN-L"
- board text removed: "DashFault"
- board text removed: "GreenLEDS"
- board text removed: "HV"
- board text removed: "HVIL"
- board text removed: "HVSwitch"
- board text removed: "LCD"
- board text removed: "LSignal"
- board text removed: "LV"
- board text removed: "LVSwitch"
- board text removed: "ModeSelect"
- board text removed: "PreCharge"
- board text removed: "RSignal"
